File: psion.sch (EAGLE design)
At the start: 92 parts, among them J2 1-2295018-2, Q2 NTF3055L108T1G, Q3 NTF3055L108T1G, Q5 MOSFET-PCH_SOT-223, Q6 MOSFET-PCH_SOT-223, Q8 MMBT2907ALT1G, T1 2908-05WB-MG, U2 HV823LG-G, U3 ATMEGA32U4-AU, U4 OSD3358-512M-BCB, U5 MAX1620EEE+, U6 MAX1620EEE+, U7 ATTINY404-SSN, U8 TPS61090RSAR, Y1 ABM10-16.000MHZ-D30-T3

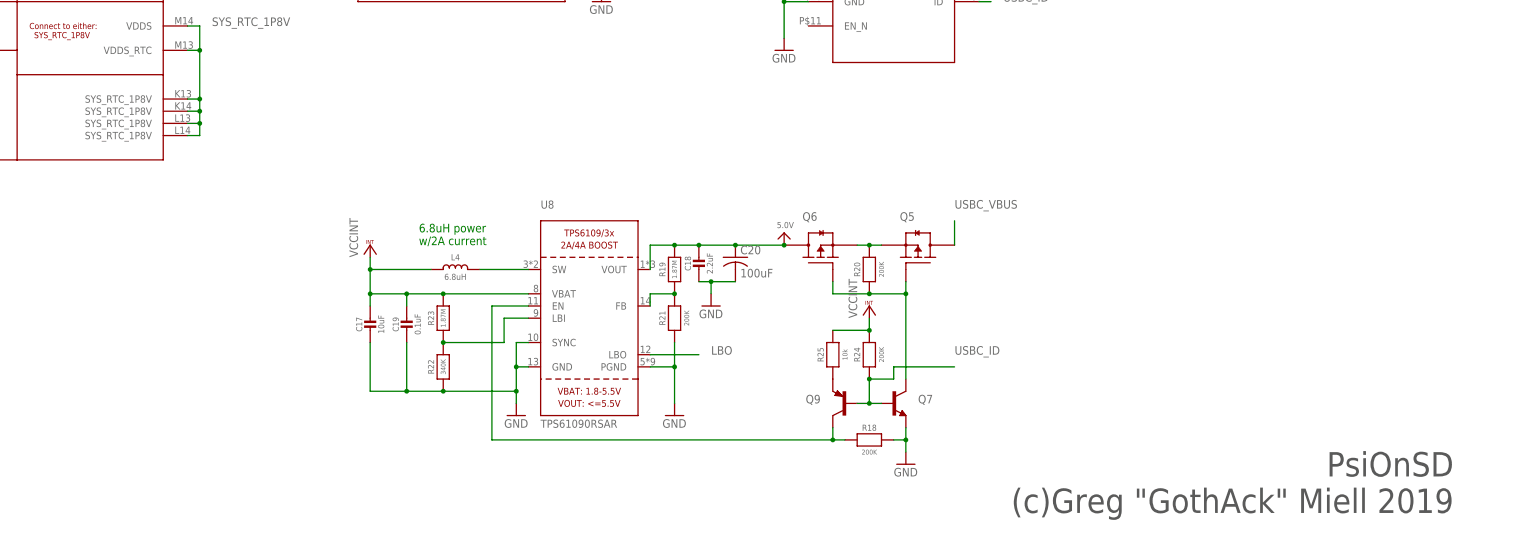
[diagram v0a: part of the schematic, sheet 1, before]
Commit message: add TAPR OHL license
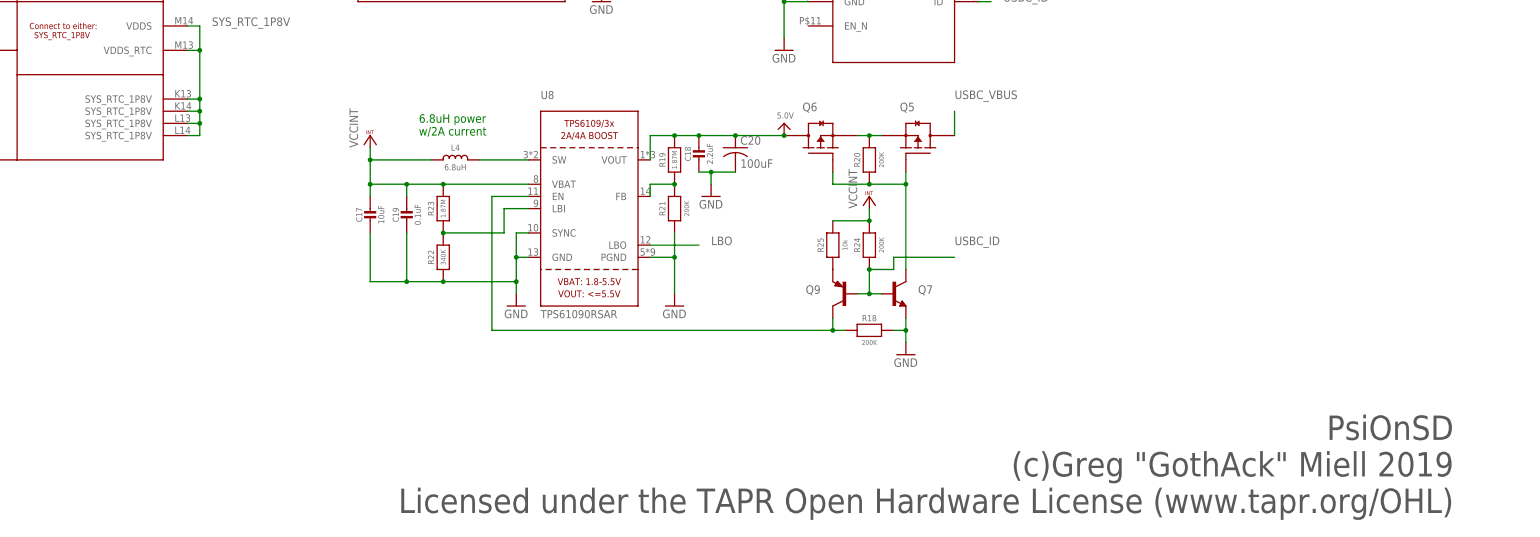
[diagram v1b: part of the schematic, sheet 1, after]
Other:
- note added: "PsiOnSD (c)Greg "GothAck" Miell 2019 Licensed under the TAPR Open Hardware License (www.tapr.org/OHL)"
- note removed: "PsiOnSD (c)Greg "GothAck" Miell 2019"
- moved on the sheet: C14, C17, C18, C19, C20, L4, Q5, Q6, Q7, Q9, R18, R19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
